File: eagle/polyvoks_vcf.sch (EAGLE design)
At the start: 52 parts, among them IC1 TL072P, IC2 LM4250P, IC3 TL071P, IC4 LM4250P, IC5 TL072P, T1 2N3904

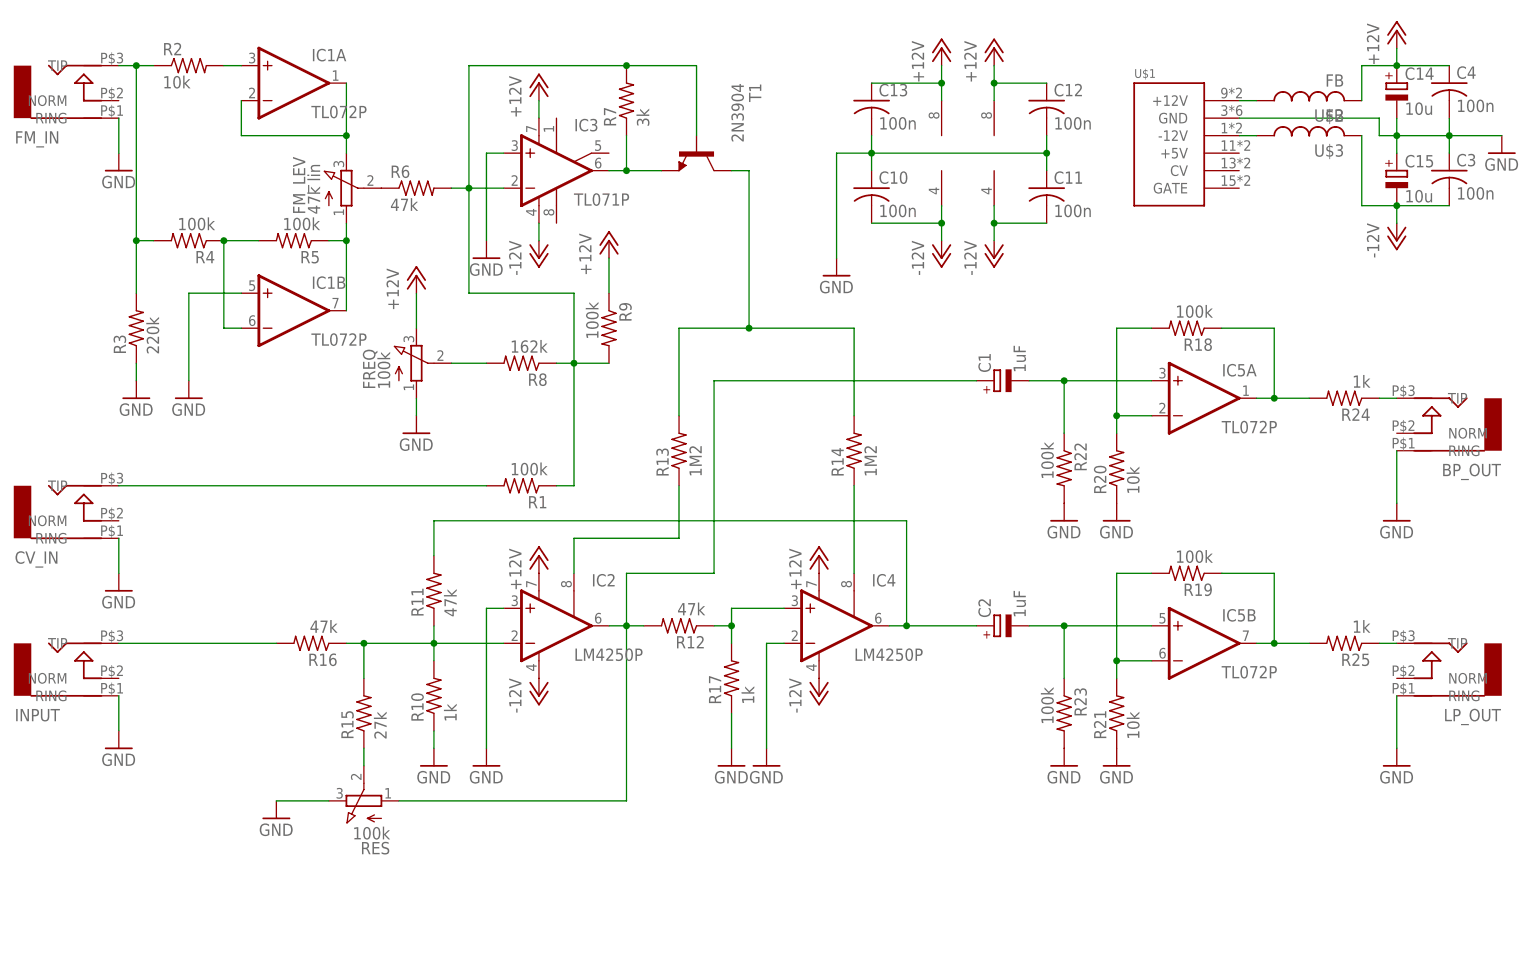
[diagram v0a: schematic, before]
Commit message: schemo modded
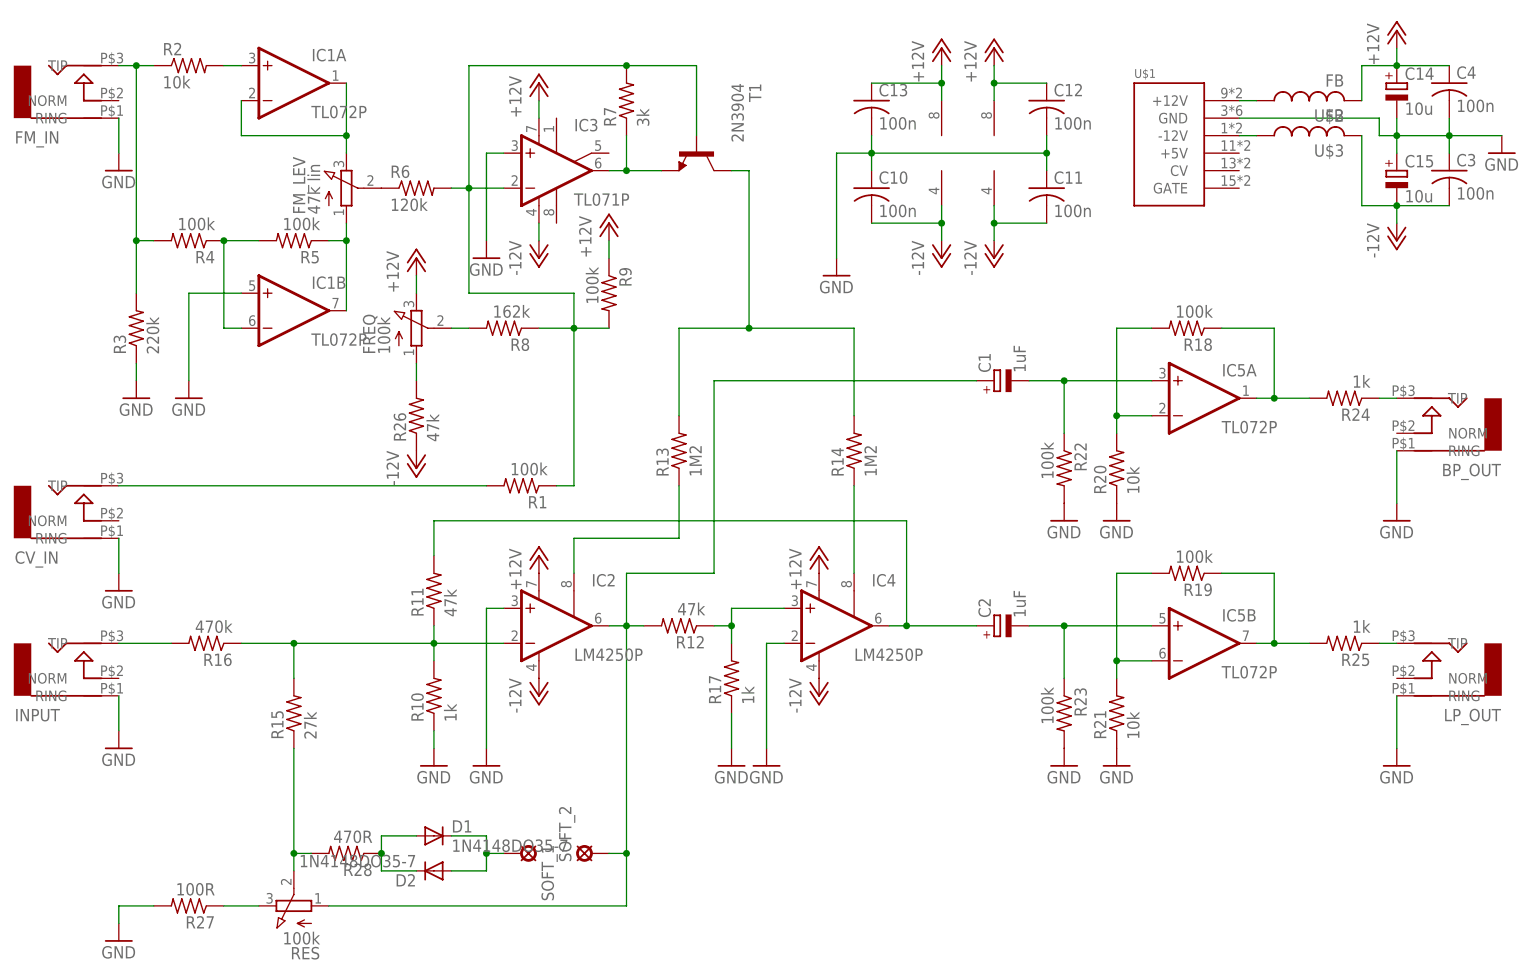
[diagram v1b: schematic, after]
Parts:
- added D1, D2: 1N4148DO35-7, diode:1N4148DO35-7
- added R26: 47k, rcl:R-US_0207/10
- added R27: 100R, rcl:R-US_0207/10
- added R28: 470R, rcl:R-US_0207/10
- added SOFT_1, SOFT_2: LSP11, solpad:LSP11
- R16: value 47k -> 470k
- R6: value 47k -> 120k
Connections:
- new net GND: R27.2
- new net N$31: R27.1, RES.E
- new net N$32: D1.A, D2.C, R28.1
- new net N$33: D1.C, D2.A, SOFT_1.MP
- net -12V: now also R26.1
- net N$12: now also R28.2
- net N$13: now also SOFT_2.MP
- net N$30: now also R26.2; no longer RES.E
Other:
- moved on the sheet: FREQ, R15, R16, R8, R9, RES
